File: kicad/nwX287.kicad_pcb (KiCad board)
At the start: 2 copper layers, 52.5 x 24 mm, 4 parts, among them U1 bq3285, U2 Socket, Y1 32.768kHz 6pF

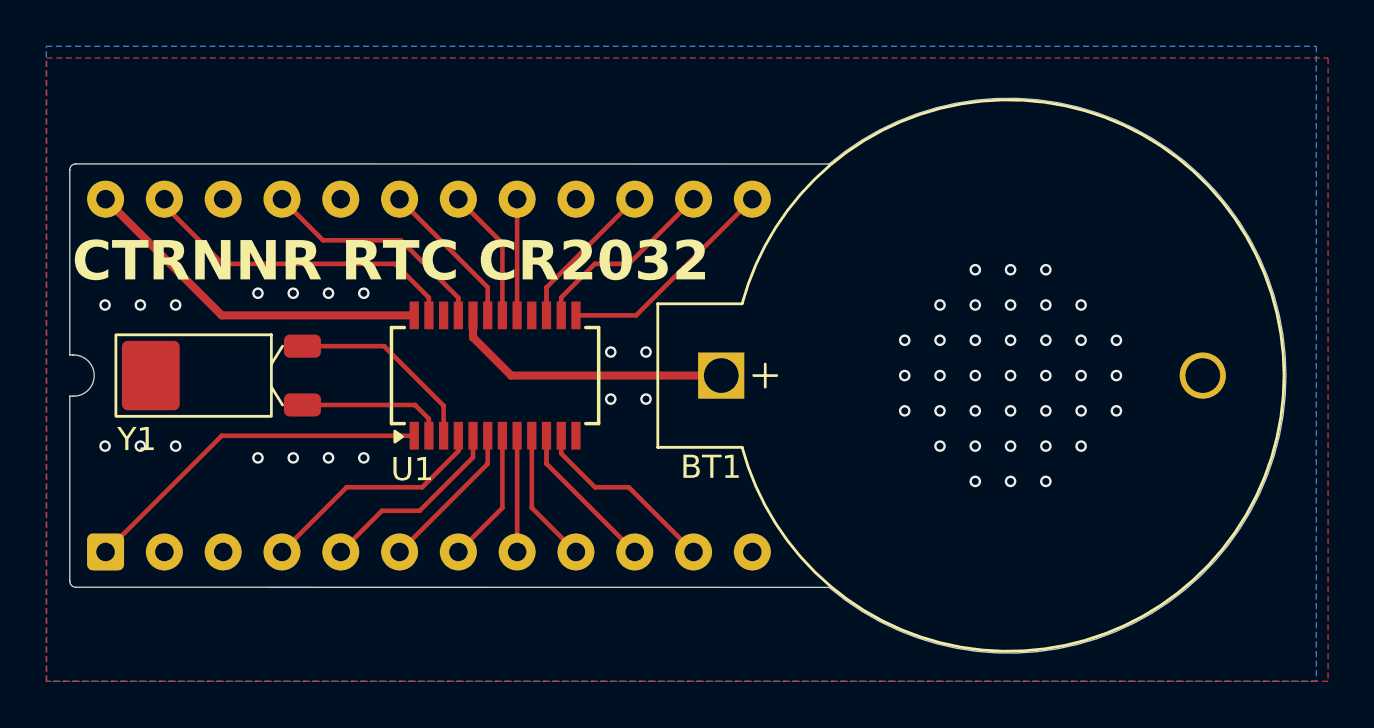
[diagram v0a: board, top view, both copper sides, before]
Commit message: adjust tracks
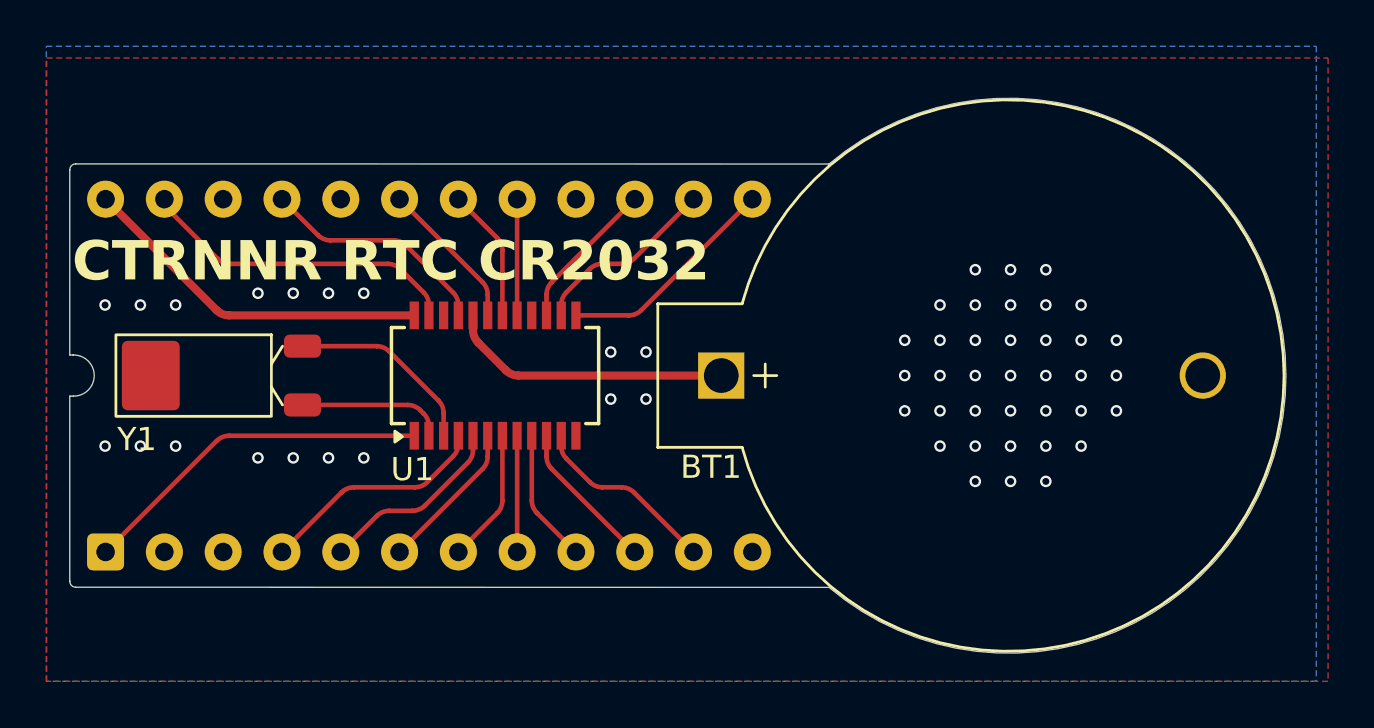
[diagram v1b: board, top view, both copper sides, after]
